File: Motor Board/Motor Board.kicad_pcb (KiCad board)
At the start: 2 copper layers, 37.5 x 39 mm, 30 parts, among them J1 Programmer, J2 Gecko, J3 Gecko, J4 Conn_01x02_Socket, J5 Conn_01x02_Socket, Q1 BSS316NN, U2 PIC18F26K83, U3 MCP2562, U4 INA180, Y1 12MHz Crystal

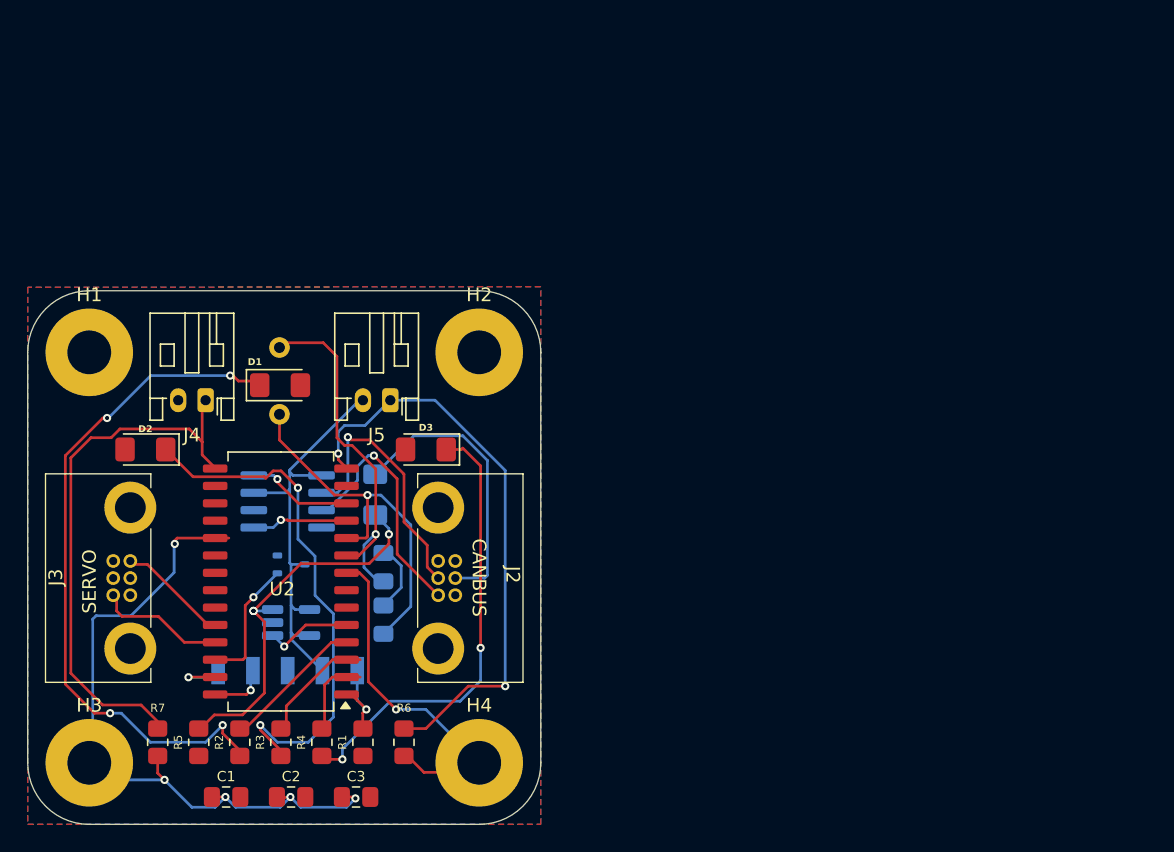
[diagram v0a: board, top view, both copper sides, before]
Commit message: Push motor
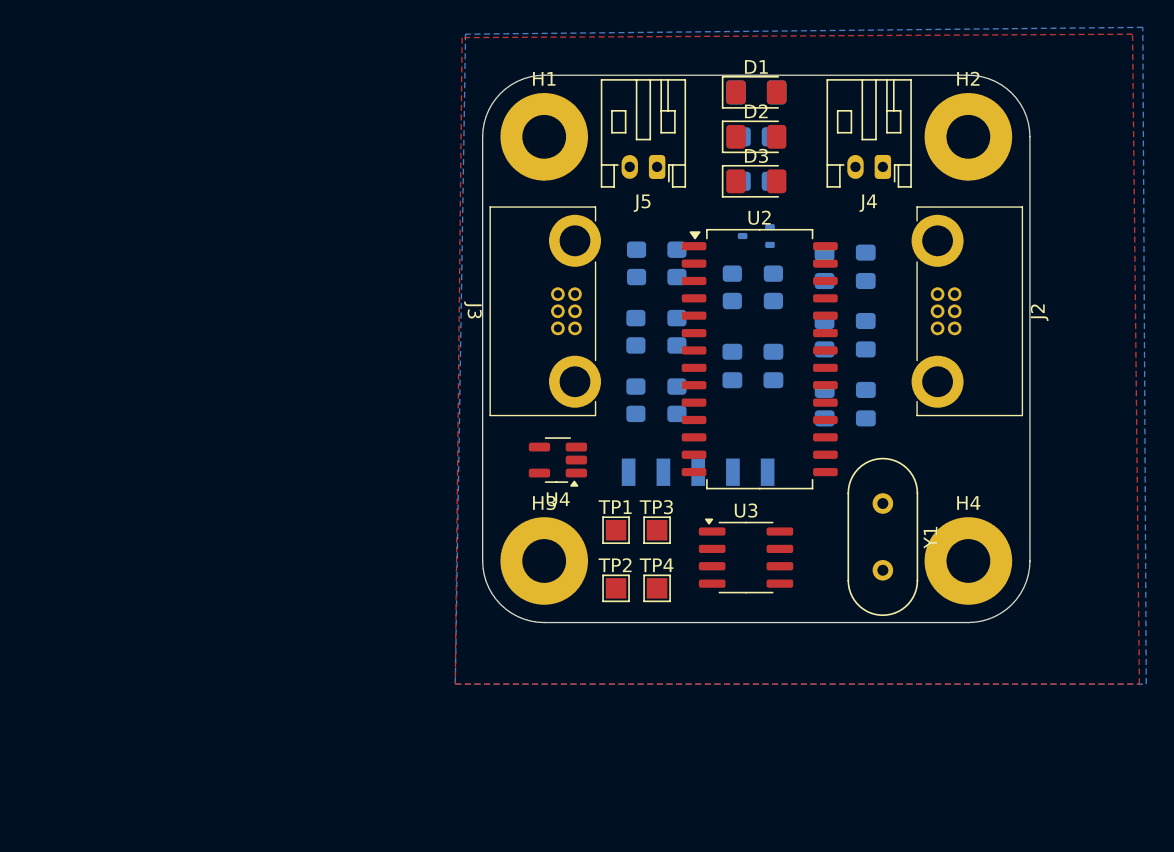
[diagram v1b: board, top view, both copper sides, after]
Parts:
- added C6: 10uF, Capacitor_SMD:C_0805_2012Metric_Pad1.18x1.45mm_HandSolder, B.Cu at (180.8, 65.3)
- added C7: 10uF, Capacitor_SMD:C_0805_2012Metric_Pad1.18x1.45mm_HandSolder, B.Cu at (171.0, 62.5)
- added C8: 10uF, Capacitor_SMD:C_0805_2012Metric_Pad1.18x1.45mm_HandSolder, B.Cu at (174.0, 62.5)
- added R10: 1kR, Resistor_SMD:R_0805_2012Metric_Pad1.20x1.40mm_HandSolder, B.Cu at (174.0, 56.8)
- added R8: 10kR, Resistor_SMD:R_0805_2012Metric_Pad1.20x1.40mm_HandSolder, B.Cu at (166.9, 65.0)
- added R9: 1kR, Resistor_SMD:R_0805_2012Metric_Pad1.20x1.40mm_HandSolder, B.Cu at (171.0, 56.8)
- added TP1: 5v TP, TestPoint:TestPoint_Pad_1.5x1.5mm, F.Cu at (162.5, 74.5)
- added TP2: PWM TP, TestPoint:TestPoint_Pad_1.5x1.5mm, F.Cu at (162.5, 78.8)
- added TP3: LIM2 TP, TestPoint:TestPoint_Pad_1.5x1.5mm, F.Cu at (165.5, 74.5)
- added TP4: LIM1 TP, TestPoint:TestPoint_Pad_1.5x1.5mm, F.Cu at (165.5, 78.8)
- C1, C2, C3, R1, R2, R3, R4, R6, R7: moved to B.Cu
- F1: value Polyfuse 350mA -> Polyfuse 750mA
- R5: value 62mR -> 10R; moved to B.Cu
- U3, U4, Y1: moved to F.Cu
- moved C1 58.4 mm to (177.7, 55.2), turned to -90 degrees
- moved C2 57.1 mm to (180.8, 55.2), turned to -90 degrees
- moved R2 55.7 mm to (172.8, 49.0), turned to 180 degrees
- moved R1 52.8 mm to (172.8, 45.8), turned to 180 degrees
- moved J4 52.4 mm to (182.0, 48.0)
- moved D2 50.2 mm to (172.8, 45.8), turned to 0 degrees
- moved C3 48.1 mm to (177.7, 60.2), turned to -90 degrees
- moved R5 46.1 mm to (166.9, 60.0), turned to -90 degrees
- moved Y1 45.5 mm to (182.0, 72.5)
- moved R3 43.6 mm to (164.0, 55.0), turned to -90 degrees
- moved R4 43.6 mm to (166.9, 55.0), turned to -90 degrees
- moved R7 43.0 mm to (163.9, 65.0)
- moved Q1 41.6 mm to (172.8, 53.0), turned to 180 degrees
- moved J2 41.4 mm to (186.0, 58.5)
- moved D1 40.9 mm to (172.8, 42.5)
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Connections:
- J3 pad 5: +5V -> Net-(J3-Pin_5)
- J4 pad 1: /LIM_2 -> GND
- J4 pad 2: +5V -> Net-(J4-Pin_2)
- J5 pad 1: /LIM_1 -> GND
- J5 pad 2: +5V -> Net-(J5-Pin_2)
- Q1 pad 2: GND -> +5V
- Q1 pad 3: +5V -> Net-(J3-Pin_5)
- R6 pad 1: /LIM_1 -> +5V
- R6 pad 2: GND -> Net-(J5-Pin_2)
- R7 pad 1: /LIM_2 -> +5V
- R7 pad 2: GND -> Net-(J4-Pin_2)
- U3 pad 2: GND -> Net-(U3-STBY)
- U3 pad 8: GND -> Net-(U3-STBY)
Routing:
- net GND: track 81.2 -> 0.00 mm, vias 6 -> 0
- net Net-(D1-K): track 50.2 -> 0.00 mm, vias 4 -> 0
- net /LIM_1: track 42.4 -> 0.00 mm, vias 2 -> 0
- net /LIM_2: track 40.6 -> 0.00 mm
- net Net-(D2-K): track 38.8 -> 0.00 mm, vias 2 -> 0
- net Net-(D3-K): track 33.1 -> 0.00 mm, vias 2 -> 0
- net +5V: track 31.2 -> 0.00 mm
- net Net-(U4-IN+): track 28.0 -> 0.00 mm, vias 3 -> 0
- net /OSC2: track 28.0 -> 0.00 mm, vias 1 -> 0
- net /OSC1: track 26.5 -> 0.00 mm, vias 1 -> 0
- net Net-(J2-Pin_5): track 20.9 -> 0.00 mm
- net /CANL: track 19.4 -> 0.00 mm, vias 1 -> 0
- net /CANH: track 17.8 -> 0.00 mm, vias 1 -> 0
- net Net-(U2-RA2): track 10.3 -> 0.00 mm
- net /MTR_ON: track 9.39 -> 0.00 mm, vias 1 -> 0
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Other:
- board size 37.5 x 39 mm -> 40 x 40 mm
- board text removed: "CANBUS"
- board text removed: "SERVO"

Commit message: Fix review items
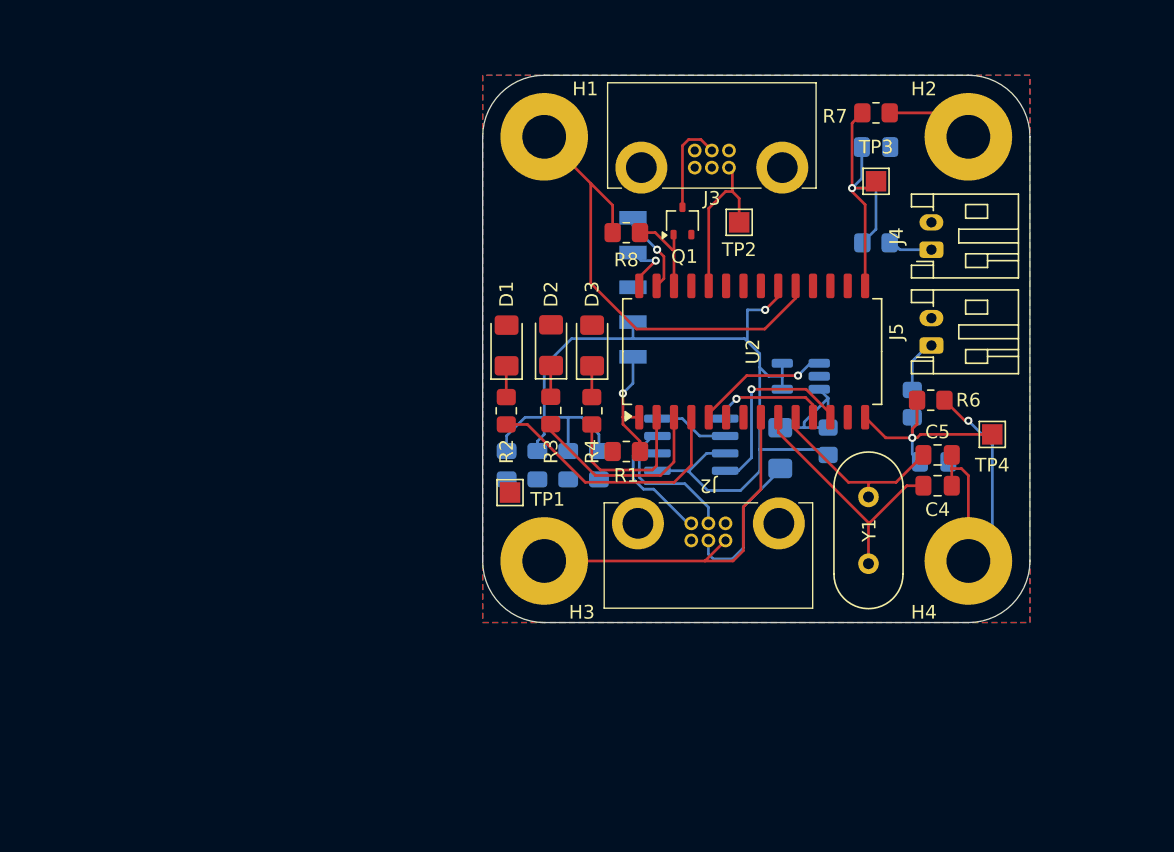
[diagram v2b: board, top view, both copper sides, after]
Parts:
- C4, C5, Q1, R1, R2, R3, R4, R6, R7, R8: moved to F.Cu
- F1: value Polyfuse 750mA -> Polyfuse 1.5A
- R5: value 10R -> 50mR
- U3, U4: moved to B.Cu
- moved TP3 30.1 mm to (181.5, 49.0)
- moved TP2 28.2 mm to (171.5, 52.0)
- moved R7 27.4 mm to (181.5, 44.0), turned to 0 degrees
- moved TP4 27.0 mm to (190.0, 67.5)
- moved C6 26.6 mm to (154.5, 69.8)
- moved F1 26.1 mm to (174.5, 68.5), turned to -90 degrees
- moved D1 26.0 mm to (154.5, 61.0), turned to 90 degrees
- moved R1 24.9 mm to (163.2, 68.8), turned to 0 degrees
- moved R2 24.8 mm to (154.5, 65.8), turned to -90 degrees
- moved C2 24.3 mm to (161.2, 69.8)
- moved J5 23.9 mm to (185.6, 61.0), turned to 90 degrees
- moved C1 23.7 mm to (159.0, 69.8)
- moved C3 23.0 mm to (156.8, 69.8), turned to 90 degrees
- moved J2 22.8 mm to (169.2, 74.0), turned to 0 degrees
- moved R6 22.1 mm to (185.5, 65.0), turned to 0 degrees
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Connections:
- C4 pad 2: Net-(C4-Pad2) -> GND
- C5 pad 2: Net-(C4-Pad2) -> GND
- J3 pad 4: /MTR_OUT -> unconnected-(J3-Pin_4-Pad4)
- J4 pad 1: GND -> Net-(J4-Pin_1)
- J4 pad 2: Net-(J4-Pin_2) -> +5V
- J5 pad 1: GND -> Net-(J5-Pin_1)
- J5 pad 2: Net-(J5-Pin_2) -> +5V
- R10 pad 1: GND -> Net-(J5-Pin_1)
- R6 pad 1: +5V -> /LIM_1
- R6 pad 2: Net-(J5-Pin_2) -> GND
- R7 pad 1: +5V -> /LIM_2
- R7 pad 2: Net-(J4-Pin_2) -> GND
- R9 pad 1: GND -> Net-(J4-Pin_1)
- U2 pad 25: /MTR_OUT -> unconnected-(U2-RB4-Pad25)
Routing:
- net GND: track 0.00 -> 92.3 mm, vias 0 -> 1
- net +5V: track 0.00 -> 72.5 mm, vias 0 -> 1
- net /LIM_2: track 0.00 -> 24.8 mm, vias 0 -> 1
- net Net-(U2-RA2): track 0.00 -> 19.3 mm
- net /OSC1: track 0.00 -> 18.6 mm
- net /LIM_1: track 0.00 -> 16.4 mm, vias 0 -> 1
- net Net-(U2-RA1): track 0.00 -> 14.5 mm
- net /CAN_RX: track 0.00 -> 14.1 mm, vias 0 -> 1
- net /OSC2: track 0.00 -> 13.8 mm
- net /MTR_IN: track 0.00 -> 12.2 mm
- net Net-(U2-RA0): track 0.00 -> 11.4 mm
- net Net-(J2-Pin_5): track 0.00 -> 11.0 mm
- net /CANL: track 0.00 -> 10.0 mm
- net /CURR_SENS: track 0.00 -> 9.87 mm, vias 0 -> 1
- net /CANH: track 0.00 -> 9.67 mm
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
